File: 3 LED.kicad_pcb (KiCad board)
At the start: 2 copper layers, 24 x 48 mm, 15 parts, among them J1 Conn_01x04_Socket, Q1 NPN, Q2 NPN, Q3 NPN, U1 74HC238

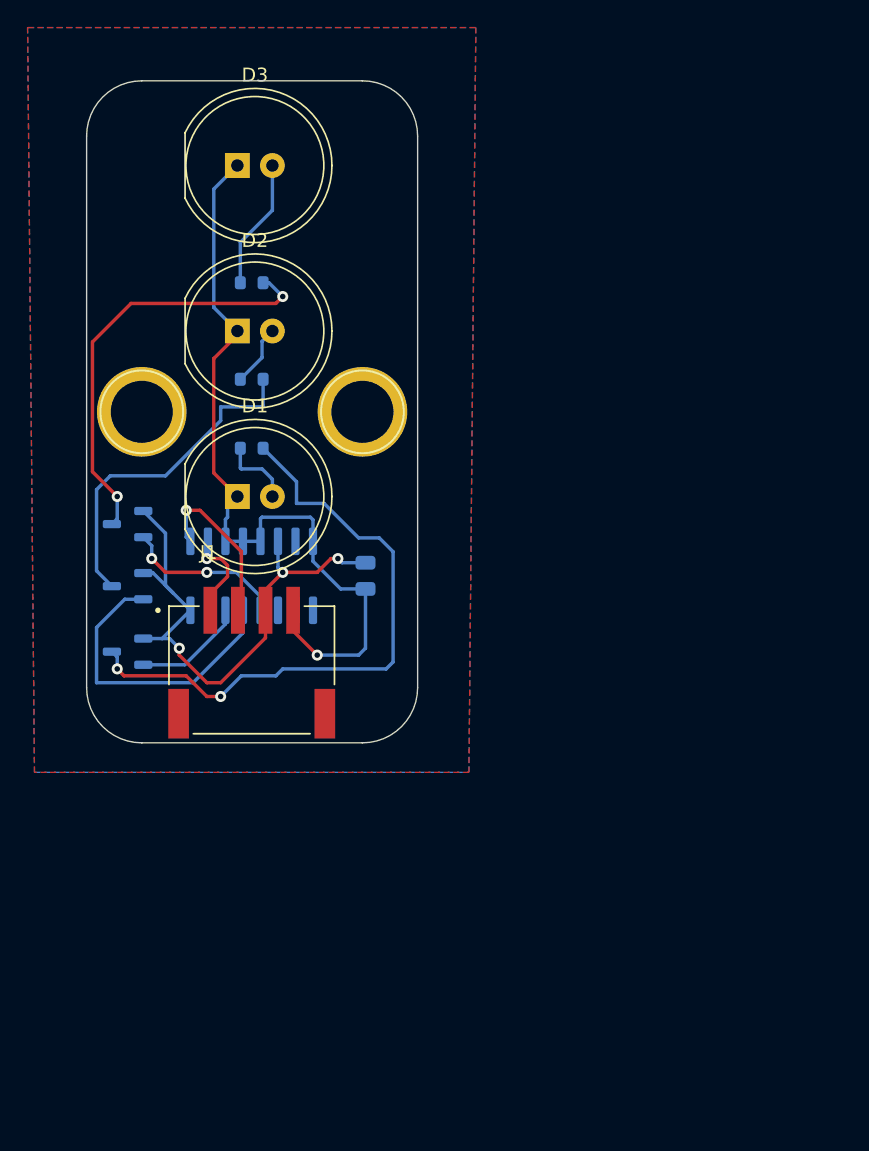
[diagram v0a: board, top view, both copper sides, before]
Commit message: update Schematic
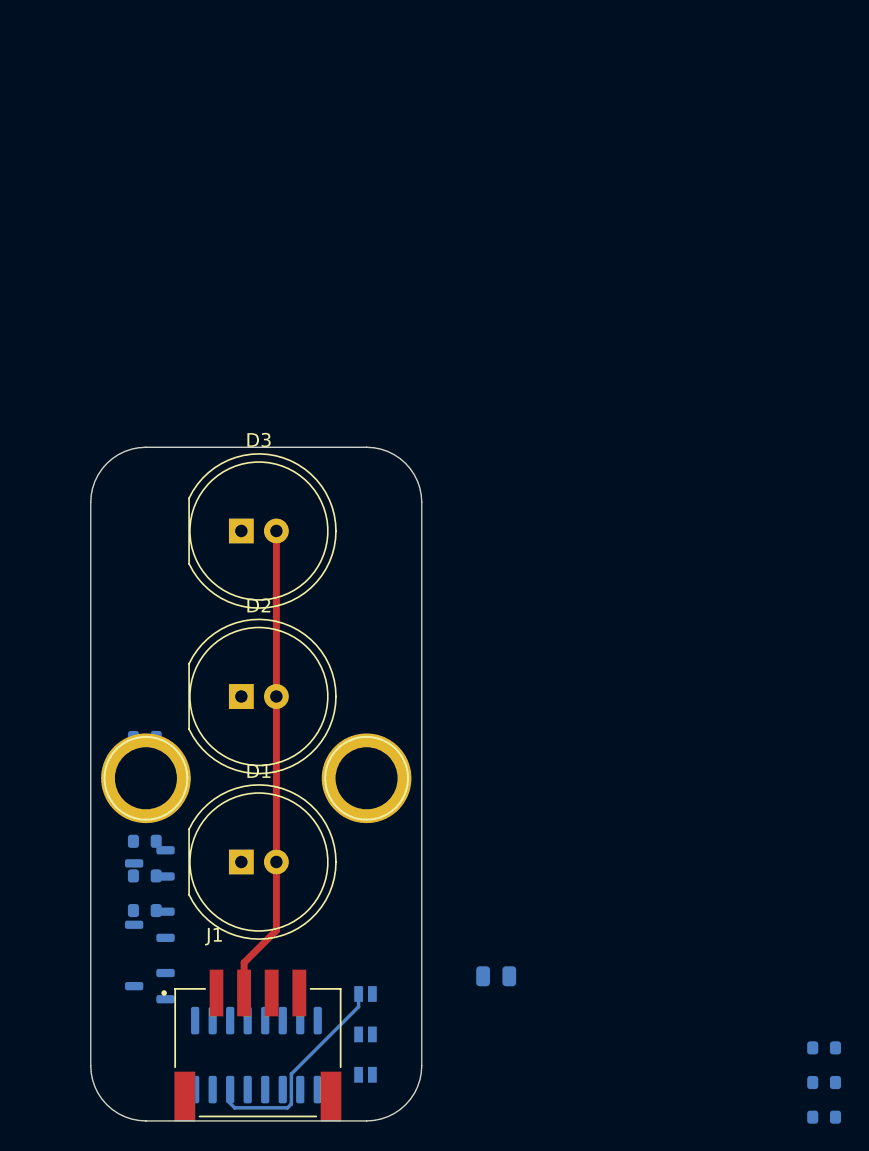
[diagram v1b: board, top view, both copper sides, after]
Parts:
- removed G***: LOGO, DeltaKiteEngineering:BKU_Medium
- removed G***: LOGO, DeltaKiteEngineering:DeltaKite_Large
- removed the REF** at (142.2, 111.8)
- added JP1: Jumper_2_Open, SofleRGB:Jumper, B.Cu at (149.5, 125.6)
- added JP2: Jumper_2_Open, SofleRGB:Jumper, B.Cu at (149.5, 128.5)
- added JP3: Jumper_2_Open, SofleRGB:Jumper, B.Cu at (149.5, 131.4)
- added R4: R, Resistor_SMD:R_0603_1608Metric, B.Cu at (182.8, 129.5)
- added R5: R, Resistor_SMD:R_0603_1608Metric, B.Cu at (182.8, 132.0)
- added R6: R, Resistor_SMD:R_0603_1608Metric, B.Cu at (182.8, 134.5)
- added R7: R, Resistor_SMD:R_0603_1608Metric, B.Cu at (133.5, 114.5)
- added R8: R, Resistor_SMD:R_0603_1608Metric, B.Cu at (133.5, 117.0)
- added R9: R, Resistor_SMD:R_0603_1608Metric, B.Cu at (133.5, 119.5)
- added REF**: Ohstem_Base, ACLAB:Ohstem_Base, F.Cu at (142.5, 116.0)
- U1: value 74HC238 -> 74HC238D
- moved R3 38.8 mm to (133.5, 112.0)
- moved U1 34.8 mm to (141.6, 130.0)
- moved Q3 33.5 mm to (133.9, 125.0)
- moved C1 30.5 mm to (159.0, 124.3), turned to 180 degrees
- moved R2 29.5 mm to (133.5, 109.5)
- moved J1 27.8 mm to (141.7, 129.8)
- moved D1 26.5 mm to (140.5, 116.0)
- moved D2 26.5 mm to (140.5, 104.0)
- moved D3 26.5 mm to (140.5, 92.0)
- moved Q2 24.6 mm to (133.9, 120.5)
- moved R1 22.4 mm to (133.5, 107.0)
- moved Q1 15.4 mm to (133.9, 116.1)
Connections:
- D1 pad 1: GND -> Net-(D1-K)
- D1 pad 2: Net-(D1-A) -> +5V
- D2 pad 1: GND -> Net-(D2-K)
- D2 pad 2: Net-(D2-A) -> +5V
- D3 pad 1: GND -> Net-(D3-K)
- D3 pad 2: Net-(D3-A) -> +5V
- J1 pad 1: /S1 -> GND
- J1 pad 2: /S0 -> +5V
- J1 pad 3: +5V -> /S1
- J1 pad 4: GND -> /S0
- Q1 pad 1: +5V -> Net-(JP1-A)
- Q1 pad 2: /L1 -> Net-(Q1-B)
- Q1 pad 3: Net-(Q1-E) -> GND
- Q2 pad 1: +5V -> Net-(JP2-A)
- Q2 pad 2: /L2 -> Net-(Q2-B)
- Q2 pad 3: Net-(Q2-E) -> GND
- Q3 pad 1: +5V -> Net-(JP3-B)
- Q3 pad 2: /L3 -> Net-(Q3-B)
- Q3 pad 3: Net-(Q3-E) -> GND
- R1 pad 1: Net-(Q1-E) -> Net-(D1-K)
- R1 pad 2: Net-(D1-A) -> Net-(JP1-A)
- R2 pad 1: Net-(Q2-E) -> Net-(D2-K)
- R2 pad 2: Net-(D2-A) -> Net-(JP2-A)
- R3 pad 1: Net-(Q3-E) -> Net-(D3-K)
- R3 pad 2: Net-(D3-A) -> Net-(JP3-B)
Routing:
- net GND: track 58.2 -> 0.00 mm, vias 1 -> 0
- net Net-(Q1-E): track 44.7 -> 0.00 mm, vias 2 -> 0
- net Net-(Q3-E): track 31.1 -> 0.00 mm, vias 2 -> 0
- net Net-(Q2-E): track 24.6 -> 0.00 mm
- net /L2: track 22.0 -> 0.00 mm
- net /S0: track 12.0 -> 0.00 mm, vias 1 -> 0
- net /L3: track 11.8 -> 0.00 mm, vias 2 -> 0
- net Net-(D3-A): track 9.46 -> 0.00 mm
- net /L1: track 8.18 -> 15.7 mm
- net /S1: track 6.76 -> 0.00 mm, vias 1 -> 0
- net +5V: track 40.3 -> 34.5 mm, vias 3 -> 0
- net Net-(D1-A): track 5.34 -> 0.00 mm
- net Net-(D2-A): track 4.46 -> 0.00 mm
- removed copper zone on B.Cu, net GND
- removed copper zone on F.Cu, net GND
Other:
- board size 24 x 48 mm -> 24 x 48.8 mm
